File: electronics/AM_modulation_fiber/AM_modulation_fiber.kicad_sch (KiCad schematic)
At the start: 4 parts

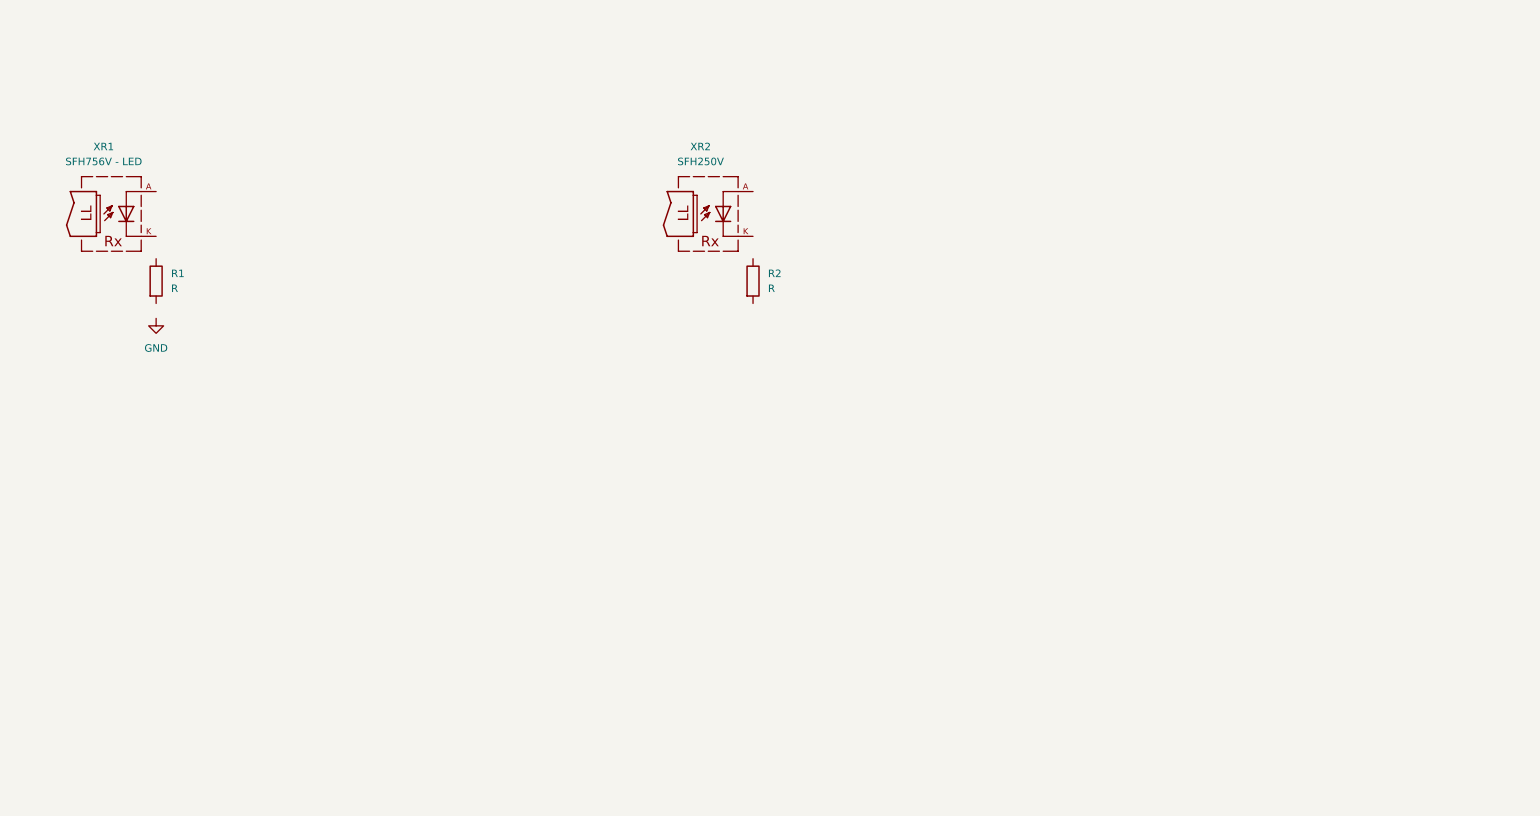
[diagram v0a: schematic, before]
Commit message: Update AM_modulation_filter
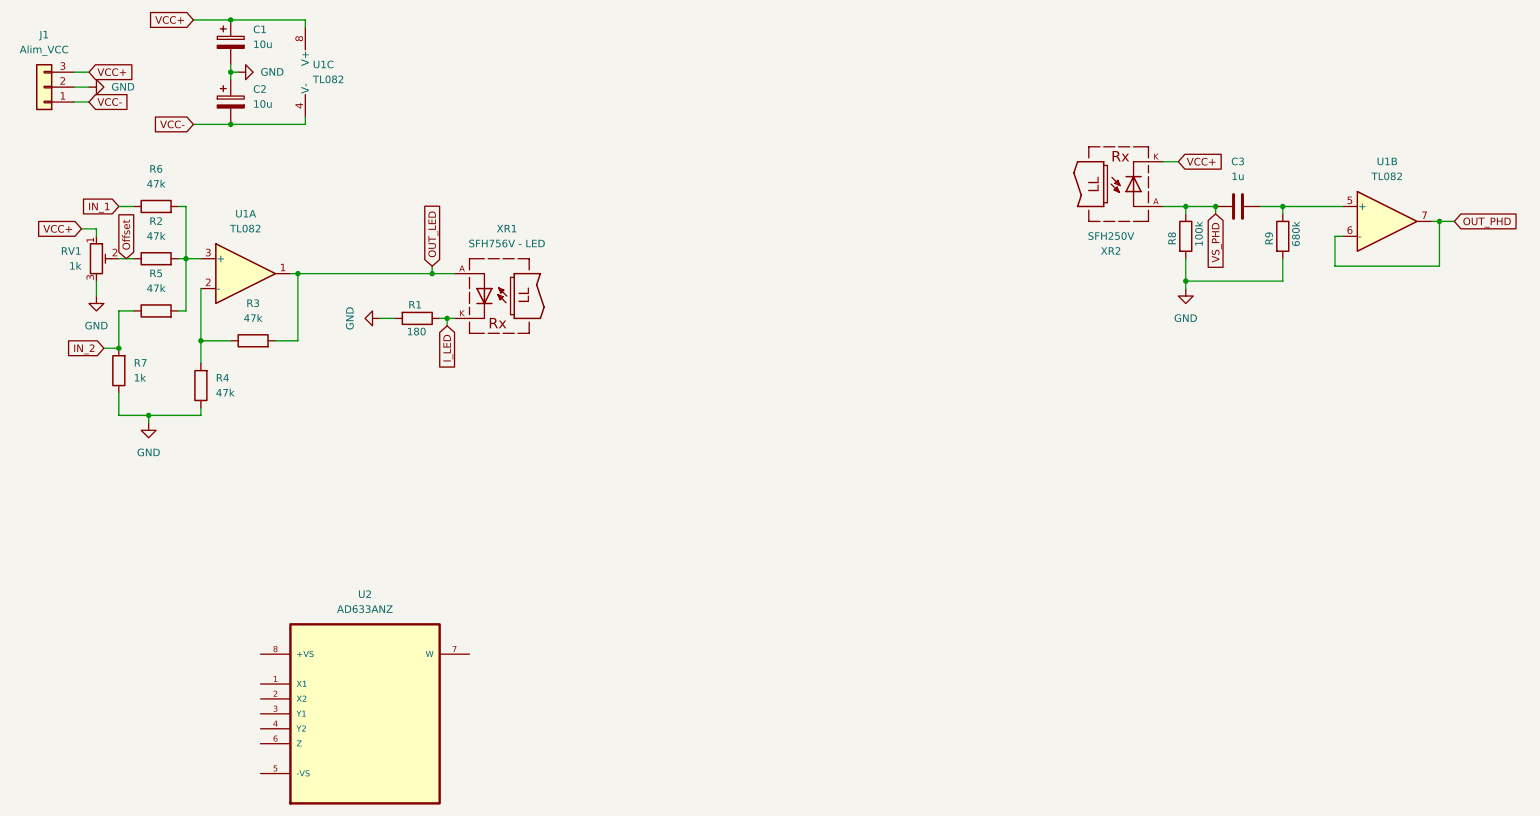
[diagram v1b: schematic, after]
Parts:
- added C1, C2: 10u, symbol Device:C_Polarized
- added C3: 1u, symbol Device:C
- added J1: Alim_VCC, symbol Connector_Generic:Conn_01x03
- added R3, R4, R5, R6: 47k, Resistor_THT:R_Axial_DIN0207_L6.3mm_D2.5mm_P10.16mm_Horizontal, symbol Device:R
- added R7: 1k, Resistor_THT:R_Axial_DIN0207_L6.3mm_D2.5mm_P10.16mm_Horizontal, symbol Device:R
- added R8: 100k, Resistor_THT:R_Axial_DIN0207_L6.3mm_D2.5mm_P10.16mm_Horizontal, symbol Device:R
- added R9: 680k, Resistor_THT:R_Axial_DIN0207_L6.3mm_D2.5mm_P10.16mm_Horizontal, symbol Device:R
- added RV1: 1k, symbol Device:R_Potentiometer_Trim
- added U1: TL082, symbol Amplifier_Operational:TL082
- added U2: AD633ANZ, AD633ANZ:DIP254P762X533-8, symbol AD633ANZ:AD633ANZ
- R1: value R -> 180
- R2: value R -> 47k
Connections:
- net GND: now also R1.2, C1.2, C2.1, J1.2 (Pin_2), R4.1, R7.1, R8.2, R9.2, RV1.3
- net OUT_LED: now reaches XR1.A
- net OUT_LED: now also R3.2, U1.1
- net I_LED: now reaches XR1.K
- net I_LED: now also R1.1
- net VS_PHD: now reaches XR2.A
- net VS_PHD: now also C3.1, R8.1
- net VCC+: now reaches XR2.K
- net VCC+: now also C1.1, J1.3 (Pin_3), RV1.1, U1.8 (V+)
- net Offset: now reaches R2.1
- net Offset: now also RV1.2
- net at R2.2: now also R5.2, R6.2, U1.3 (+)
- new net: R3.1, R4.2, U1.2 (-)
- new net: C3.2, R9.1, U1.5 (+)
- new net IN_1: R6.1
- new net IN_2: R5.1, R7.2
- new net OUT_PHD: U1.6 (-), U1.7
- new net VCC-: C2.2, J1.1 (Pin_1), U1.4 (V-)
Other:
- moved on the sheet: R1, XR1, XR2
